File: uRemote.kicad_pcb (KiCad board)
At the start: 4 copper layers, 50 x 70 mm, 44 parts, among them J2 USB_B_Micro, SW1 Rotary_Encoder_Switch, U1 74HC14, U2 FT230XS, U3 LTC4054XES5-4.2, U4 STM32L011D4Px

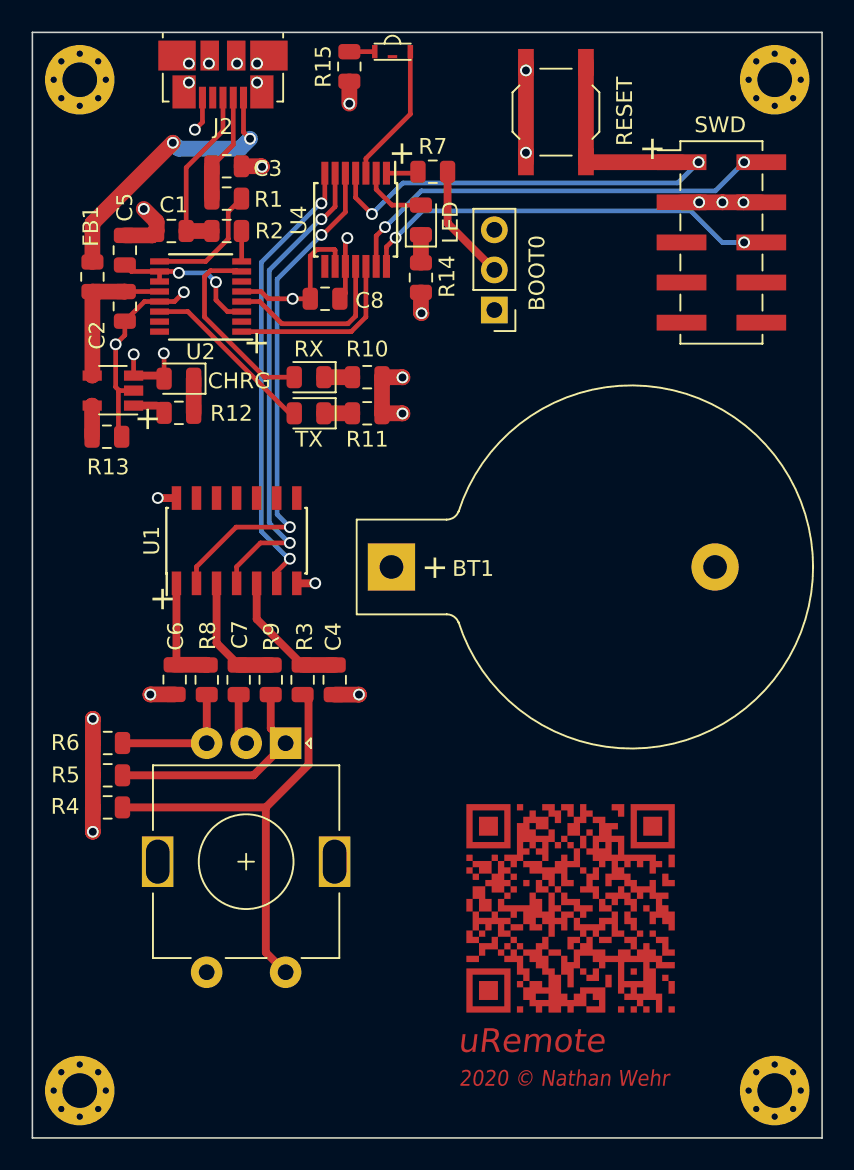
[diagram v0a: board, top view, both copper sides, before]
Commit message: WIP
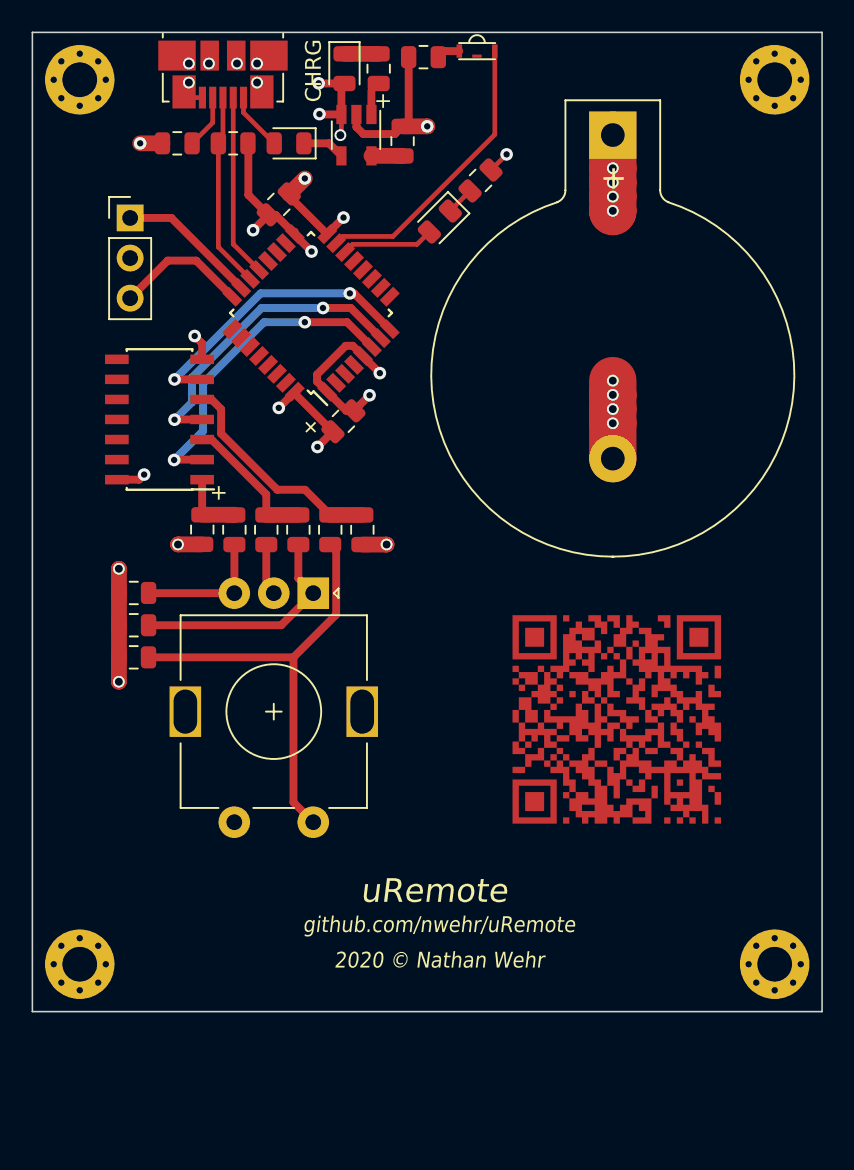
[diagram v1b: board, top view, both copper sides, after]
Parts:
- removed BOOT0: Jumper_3_Open, Connector_PinHeader_2.54mm:PinHeader_1x03_P2.54mm_Vertical
- removed C3: 47pF, Capacitor_SMD:C_0805_2012Metric
- removed C5: .1uF, Capacitor_SMD:C_0805_2012Metric
- removed C8: .01uF, Capacitor_SMD:C_0805_2012Metric
- removed FB1: Ferrite_Bead_Small, Inductor_SMD:L_0805_2012Metric
- removed LED, RX, TX: LED, LED_SMD:LED_0805_2012Metric
- removed R10, R11: 2K2, Resistor_SMD:R_0805_2012Metric
- removed R7: 10K, Resistor_SMD:R_0805_2012Metric
- removed RESET: SW_Push, Button_Switch_SMD:SW_SPST_TL3342
- removed SWD: Conn_02x05_Odd_Even, Connector_PinHeader_2.54mm:PinHeader_2x05_P2.54mm_Vertical_SMD
- removed U4: STM32L011D4Px, Package_SO:TSSOP-14_4.4x5mm_P0.65mm
- added D1: D, Diode_SMD:D_0805_2012Metric, F.Cu at (36.2, 27.0)
- added J1: Conn_01x03_Male, Connector_PinHeader_2.54mm:PinHeader_1x03_P2.54mm_Vertical, F.Cu at (26.2, 31.8)
- added LED1: LED, LED_SMD:LED_0805_2012Metric, F.Cu at (45.8, 32.0)
- C1: value 47pF -> .01uF
- R1, R2: value 27R -> 100K
- U2: value FT230XS -> STM32L072KZTx; footprint Package_SO:SSOP-16_3.9x4.9mm_P0.635mm -> Package_QFP:LQFP-32_7x7mm_P0.8mm
- moved BT1 30.7 mm to (56.8, 26.5), turned to 270 degrees
- moved R13 26.5 mm to (43.4, 26.9), turned to 90 degrees
- moved R12 25.2 mm to (41.9, 22.3), turned to 270 degrees
- moved U3 22.3 mm to (40.5, 26.5), turned to 270 degrees
- moved CHRG 22.3 mm to (39.8, 22.3), turned to 270 degrees
- moved C1 16.2 mm to (39.7, 44.6), turned to 225 degrees
- moved QR***** 12.3 mm to (57.0, 63.5)
- moved C2 11.7 mm to (35.6, 30.9), turned to 45 degrees
- moved C4 9.66 mm to (40.9, 51.5)
- moved C6 9.66 mm to (30.8, 51.5)
- moved C7 9.66 mm to (34.8, 51.5)
- moved R3 9.66 mm to (38.9, 51.5)
- moved R8 9.66 mm to (32.8, 51.5)
- moved R9 9.66 mm to (36.8, 51.5)
- moved SW1 9.66 mm to (37.8, 55.5)
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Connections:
- net Net-(U2-Pad2) renamed OSC_IN
- BT1 pad 1: VCC -> +3V3
- C1 pad 1: GND -> +3V3
- C1 pad 2: D+ -> GND
- C2 pad 1: VBUS -> +3V3
- CHRG pad 2: VCC -> +3V3
- J2 pad 1: Net-(FB1-Pad1) -> VBUS
- R1 pad 1: Net-(R1-Pad1) -> GND
- R1 pad 2: D- -> Net-(J2-Pad4)
- R2 pad 2: Net-(R2-Pad2) -> +3V3
- R4 pad 1: VCC -> +3V3
- R5 pad 1: VCC -> +3V3
- R6 pad 1: VCC -> +3V3
- U1 pad 14: VCC -> +3V3
- U2 pad 1: RX -> +3V3
- U2 pad 10: Net-(C5-Pad1) -> Net-(U2-Pad10)
- U2 pad 11: Net-(C5-Pad1) -> Net-(U2-Pad11)
- U2 pad 12: VBUS -> Net-(U2-Pad12)
- U2 pad 13: GND -> Net-(U2-Pad13)
- U2 pad 14: TXLED -> LED
- U2 pad 15: Net-(U2-Pad15) -> IRLED
- U2 pad 16: Net-(U2-Pad16) -> GND
- U2 pad 3: Net-(C5-Pad1) -> OSC_OUT
- U2 pad 4: TX -> RST
- U2 pad 5: GND -> +3V3
- U2 pad 6: Net-(U2-Pad6) -> ChanB
- U2 pad 7: RXLED -> ChanA
- U2 pad 8: Net-(R2-Pad2) -> Button
- U2 pad 9: Net-(R1-Pad1) -> Net-(U2-Pad9)
- U3 pad 3: VCC -> +3V3
- U3 pad 4: VBUS -> +5V
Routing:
- net +3V3: track 0.00 -> 40.3 mm, vias 0 -> 14
- net RST: track 37.4 -> 0.00 mm, vias 2 -> 0
- net SWDIO: track 27.2 -> 8.87 mm, vias 2 -> 0
- net Net-(FB1-Pad1): track 17.7 -> 0.00 mm, vias 2 -> 0
- net VCC: track 17.4 -> 0.00 mm, vias 6 -> 0
- net SWCLK: track 25.7 -> 8.40 mm, vias 2 -> 0
- net GND: track 57.1 -> 41.0 mm, vias 24 -> 20
- net RXLED: track 12.3 -> 0.00 mm
- net ChanB: track 32.6 -> 20.3 mm
- net RX: track 11.5 -> 0.00 mm
- net ChanA: track 30.8 -> 19.5 mm
- net TXLED: track 11.2 -> 0.00 mm
- net TX: track 11.1 -> 0.00 mm
- net Button: track 28.8 -> 18.6 mm
- net Net-(C5-Pad1): track 9.92 -> 0.00 mm, vias 2 -> 0
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- added copper zone on In1.Cu, net +3V3
- removed copper zone on In1.Cu, net VCC
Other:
- board size 50 x 70 mm -> 50 x 62 mm
- board text added: "github.com/nwehr/uRemote"
